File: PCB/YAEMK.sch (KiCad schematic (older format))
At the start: 81 parts, among them SW1 ALPS EC11

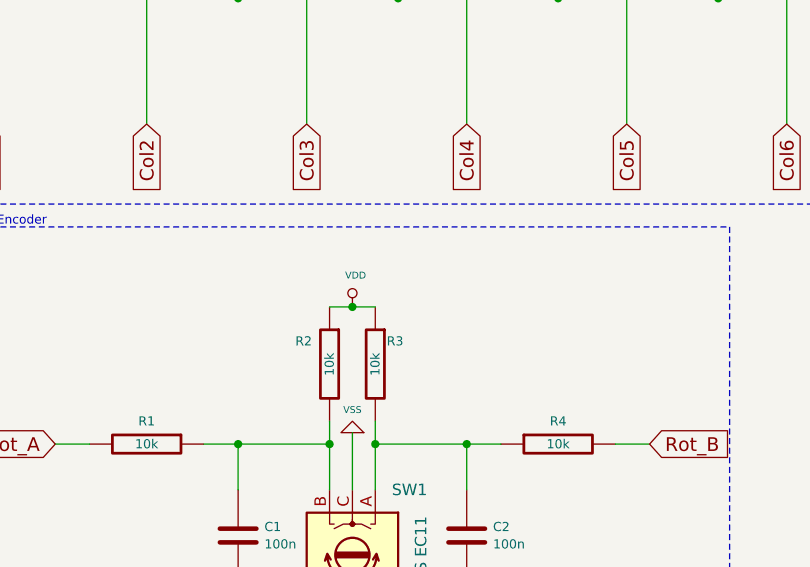
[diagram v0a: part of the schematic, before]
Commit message: YAEMK 1.2 RC
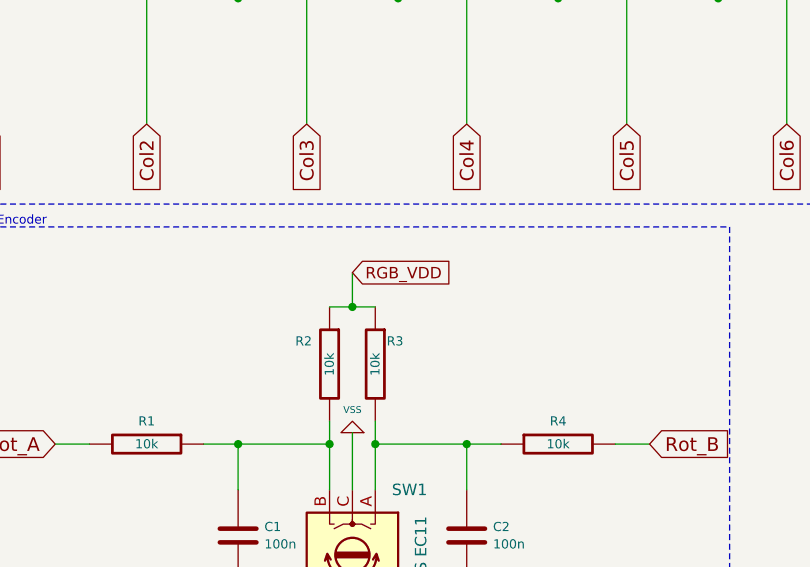
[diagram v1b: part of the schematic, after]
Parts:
- D1, D10, D11, D12, D13, D14, D15, D16, D17, D18, D19, D2, D20, D21, D22, D23, D24, D25, D26, D27, D28, D29, D3, D30, D31, D32, D33, D34, D4, D5, D6, D7, D8, D9: footprint Diode_SMD:D_SOD-523 -> prettylib:D_SOD-523
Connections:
- net VDD renamed RGB_VDD
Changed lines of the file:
@@
 F 0 "D3" H 1800 1150 40  0000 C CNN
 F 1 "DIODE" H 1800 950 40  0000 C CNN
-F 2 "Diode_SMD:D_SOD-523" H 1800 1050 60  0001 C CNN
+F 2 "prettylib:D_SOD-523" H 1800 1050 60  0001 C CNN
 F 3 "~" H 1800 1050 60  0000 C CNN
 	1    1800 1050
@@
 F 0 "D8" H 2500 1150 40  0000 C CNN
 F 1 "DIODE" H 2500 950 40  0000 C CNN
-F 2 "Diode_SMD:D_SOD-523" H 2500 1050 60  0001 C CNN
+F 2 "prettylib:D_SOD-523" H 2500 1050 60  0001 C CNN
 F 3 "~" H 2500 1050 60  0000 C CNN
 	1    2500 1050
@@
 F 0 "D13" H 3200 1150 40  0000 C CNN
 F 1 "DIODE" H 3200 950 40  0000 C CNN
-F 2 "Diode_SMD:D_SOD-523" H 3200 1050 60  0001 C CNN
+F 2 "prettylib:D_SOD-523" H 3200 1050 60  0001 C CNN
 F 3 "~" H 3200 1050 60  0000 C CNN
 	1    3200 1050
@@
 F 0 "D18" H 3900 1150 40  0000 C CNN
 F 1 "DIODE" H 3900 950 40  0000 C CNN
-F 2 "Diode_SMD:D_SOD-523" H 3900 1050 60  0001 C CNN
+F 2 "prettylib:D_SOD-523" H 3900 1050 60  0001 C CNN
 F 3 "~" H 3900 1050 60  0000 C CNN
 	1    3900 1050
@@
 F 0 "D23" H 4600 1150 40  0000 C CNN
 F 1 "DIODE" H 4600 950 40  0000 C CNN
-F 2 "Diode_SMD:D_SOD-523" H 4600 1050 60  0001 C CNN
+F 2 "prettylib:D_SOD-523" H 4600 1050 60  0001 C CNN
 F 3 "~" H 4600 1050 60  0000 C CNN
 	1    4600 1050
@@
 F 0 "D27" H 5300 1150 40  0000 C CNN
 F 1 "DIODE" H 5300 950 40  0000 C CNN
-F 2 "Diode_SMD:D_SOD-523" H 5300 1050 60  0001 C CNN
+F 2 "prettylib:D_SOD-523" H 5300 1050 60  0001 C CNN
 F 3 "~" H 5300 1050 60  0000 C CNN
 	1    5300 1050
@@
 F 0 "D31" H 6000 1150 40  0000 C CNN
 F 1 "DIODE" H 6000 950 40  0000 C CNN
-F 2 "Diode_SMD:D_SOD-523" H 6000 1050 60  0001 C CNN
+F 2 "prettylib:D_SOD-523" H 6000 1050 60  0001 C CNN
 F 3 "~" H 6000 1050 60  0000 C CNN
 	1    6000 1050
@@
 F 0 "D4" H 1800 1850 40  0000 C CNN
 F 1 "DIODE" H 1800 1650 40  0000 C CNN
-F 2 "Diode_SMD:D_SOD-523" H 1800 1750 60  0001 C CNN
+F 2 "prettylib:D_SOD-523" H 1800 1750 60  0001 C CNN
 F 3 "~" H 1800 1750 60  0000 C CNN
 	1    1800 1750
@@
 F 0 "D9" H 2500 1850 40  0000 C CNN
 F 1 "DIODE" H 2500 1650 40  0000 C CNN
-F 2 "Diode_SMD:D_SOD-523" H 2500 1750 60  0001 C CNN
+F 2 "prettylib:D_SOD-523" H 2500 1750 60  0001 C CNN
 F 3 "~" H 2500 1750 60  0000 C CNN
 	1    2500 1750
@@
 F 0 "D14" H 3200 1850 40  0000 C CNN
 F 1 "DIODE" H 3200 1650 40  0000 C CNN
-F 2 "Diode_SMD:D_SOD-523" H 3200 1750 60  0001 C CNN
+F 2 "prettylib:D_SOD-523" H 3200 1750 60  0001 C CNN
 F 3 "~" H 3200 1750 60  0000 C CNN
 	1    3200 1750
@@
 F 0 "D19" H 3900 1850 40  0000 C CNN
 F 1 "DIODE" H 3900 1650 40  0000 C CNN
-F 2 "Diode_SMD:D_SOD-523" H 3900 1750 60  0001 C CNN
+F 2 "prettylib:D_SOD-523" H 3900 1750 60  0001 C CNN
 F 3 "~" H 3900 1750 60  0000 C CNN
 	1    3900 1750
@@
 F 0 "D24" H 4600 1850 40  0000 C CNN
 F 1 "DIODE" H 4600 1650 40  0000 C CNN
-F 2 "Diode_SMD:D_SOD-523" H 4600 1750 60  0001 C CNN
+F 2 "prettylib:D_SOD-523" H 4600 1750 60  0001 C CNN
 F 3 "~" H 4600 1750 60  0000 C CNN
 	1    4600 1750
@@
 F 0 "D28" H 5300 1850 40  0000 C CNN
 F 1 "DIODE" H 5300 1650 40  0000 C CNN
-F 2 "Diode_SMD:D_SOD-523" H 5300 1750 60  0001 C CNN
+F 2 "prettylib:D_SOD-523" H 5300 1750 60  0001 C CNN
 F 3 "~" H 5300 1750 60  0000 C CNN
 	1    5300 1750
@@
 F 0 "D32" H 6000 1850 40  0000 C CNN
 F 1 "DIODE" H 6000 1650 40  0000 C CNN
-F 2 "Diode_SMD:D_SOD-523" H 6000 1750 60  0001 C CNN
+F 2 "prettylib:D_SOD-523" H 6000 1750 60  0001 C CNN
 F 3 "~" H 6000 1750 60  0000 C CNN
 	1    6000 1750
@@
 F 0 "D10" H 2500 2550 40  0000 C CNN
 F 1 "DIODE" H 2500 2350 40  0000 C CNN
-F 2 "Diode_SMD:D_SOD-523" H 2500 2450 60  0001 C CNN
+F 2 "prettylib:D_SOD-523" H 2500 2450 60  0001 C CNN
 F 3 "~" H 2500 2450 60  0000 C CNN
 	1    2500 2450
@@
 F 0 "D15" H 3200 2550 40  0000 C CNN
 F 1 "DIODE" H 3200 2350 40  0000 C CNN
-F 2 "Diode_SMD:D_SOD-523" H 3200 2450 60  0001 C CNN
+F 2 "prettylib:D_SOD-523" H 3200 2450 60  0001 C CNN
 F 3 "~" H 3200 2450 60  0000 C CNN
 	1    3200 2450
@@
 F 0 "D20" H 3900 2550 40  0000 C CNN
 F 1 "DIODE" H 3900 2350 40  0000 C CNN
-F 2 "Diode_SMD:D_SOD-523" H 3900 2450 60  0001 C CNN
+F 2 "prettylib:D_SOD-523" H 3900 2450 60  0001 C CNN
 F 3 "~" H 3900 2450 60  0000 C CNN
 	1    3900 2450
@@
 F 0 "D25" H 4600 2550 40  0000 C CNN
 F 1 "DIODE" H 4600 2350 40  0000 C CNN
-F 2 "Diode_SMD:D_SOD-523" H 4600 2450 60  0001 C CNN
+F 2 "prettylib:D_SOD-523" H 4600 2450 60  0001 C CNN
 F 3 "~" H 4600 2450 60  0000 C CNN
 	1    4600 2450
@@
 F 0 "D29" H 5300 2550 40  0000 C CNN
 F 1 "DIODE" H 5300 2350 40  0000 C CNN
-F 2 "Diode_SMD:D_SOD-523" H 5300 2450 60  0001 C CNN
+F 2 "prettylib:D_SOD-523" H 5300 2450 60  0001 C CNN
 F 3 "~" H 5300 2450 60  0000 C CNN
 	1    5300 2450
@@
 F 0 "D33" H 6000 2550 40  0000 C CNN
 F 1 "DIODE" H 6000 2350 40  0000 C CNN
-F 2 "Diode_SMD:D_SOD-523" H 6000 2450 60  0001 C CNN
+F 2 "prettylib:D_SOD-523" H 6000 2450 60  0001 C CNN
 F 3 "~" H 6000 2450 60  0000 C CNN
 	1    6000 2450
@@
 F 0 "D1" H 1100 3250 40  0000 C CNN
 F 1 "DIODE" H 1100 3050 40  0000 C CNN
-F 2 "Diode_SMD:D_SOD-523" H 1100 3150 60  0001 C CNN
+F 2 "prettylib:D_SOD-523" H 1100 3150 60  0001 C CNN
 F 3 "~" H 1100 3150 60  0000 C CNN
 	1    1100 3150
@@
 F 0 "D6" H 1800 3250 40  0000 C CNN
 F 1 "DIODE" H 1800 3050 40  0000 C CNN
-F 2 "Diode_SMD:D_SOD-523" H 1800 3150 60  0001 C CNN
+F 2 "prettylib:D_SOD-523" H 1800 3150 60  0001 C CNN
 F 3 "~" H 1800 3150 60  0000 C CNN
 	1    1800 3150
@@
 F 0 "D11" H 2500 3250 40  0000 C CNN
 F 1 "DIODE" H 2500 3050 40  0000 C CNN
-F 2 "Diode_SMD:D_SOD-523" H 2500 3150 60  0001 C CNN
+F 2 "prettylib:D_SOD-523" H 2500 3150 60  0001 C CNN
 F 3 "~" H 2500 3150 60  0000 C CNN
 	1    2500 3150
@@
 F 0 "D16" H 3200 3250 40  0000 C CNN
 F 1 "DIODE" H 3200 3050 40  0000 C CNN
-F 2 "Diode_SMD:D_SOD-523" H 3200 3150 60  0001 C CNN
+F 2 "prettylib:D_SOD-523" H 3200 3150 60  0001 C CNN
 F 3 "~" H 3200 3150 60  0000 C CNN
 	1    3200 3150
@@
 F 0 "D21" H 3900 3250 40  0000 C CNN
 F 1 "DIODE" H 3900 3050 40  0000 C CNN
-F 2 "Diode_SMD:D_SOD-523" H 3900 3150 60  0001 C CNN
+F 2 "prettylib:D_SOD-523" H 3900 3150 60  0001 C CNN
 F 3 "~" H 3900 3150 60  0000 C CNN
 	1    3900 3150
@@
 F 0 "D26" H 4600 3250 40  0000 C CNN
 F 1 "DIODE" H 4600 3050 40  0000 C CNN
-F 2 "Diode_SMD:D_SOD-523" H 4600 3150 60  0001 C CNN
+F 2 "prettylib:D_SOD-523" H 4600 3150 60  0001 C CNN
 F 3 "~" H 4600 3150 60  0000 C CNN
 	1    4600 3150
@@
 F 0 "D30" H 5300 3250 40  0000 C CNN
 F 1 "DIODE" H 5300 3050 40  0000 C CNN
-F 2 "Diode_SMD:D_SOD-523" H 5300 3150 60  0001 C CNN
+F 2 "prettylib:D_SOD-523" H 5300 3150 60  0001 C CNN
 F 3 "~" H 5300 3150 60  0000 C CNN
 	1    5300 3150
@@
 F 0 "D34" H 6000 3250 40  0000 C CNN
 F 1 "DIODE" H 6000 3050 40  0000 C CNN
-F 2 "Diode_SMD:D_SOD-523" H 6000 3150 60  0001 C CNN
+F 2 "prettylib:D_SOD-523" H 6000 3150 60  0001 C CNN
 F 3 "~" H 6000 3150 60  0000 C CNN
 	1    6000 3150
@@
 F 0 "D2" H 1100 3950 40  0000 C CNN
 F 1 "DIODE" H 1100 3750 40  0000 C CNN
-F 2 "Diode_SMD:D_SOD-523" H 1100 3850 60  0001 C CNN
+F 2 "prettylib:D_SOD-523" H 1100 3850 60  0001 C CNN
 F 3 "~" H 1100 3850 60  0000 C CNN
 	1    1100 3850
@@
 F 0 "D7" H 1800 3950 40  0000 C CNN
 F 1 "DIODE" H 1800 3750 40  0000 C CNN
-F 2 "Diode_SMD:D_SOD-523" H 1800 3850 60  0001 C CNN
+F 2 "prettylib:D_SOD-523" H 1800 3850 60  0001 C CNN
 F 3 "~" H 1800 3850 60  0000 C CNN
 	1    1800 3850
@@
 F 0 "D12" H 2500 3950 40  0000 C CNN
 F 1 "DIODE" H 2500 3750 40  0000 C CNN
-F 2 "Diode_SMD:D_SOD-523" H 2500 3850 60  0001 C CNN
+F 2 "prettylib:D_SOD-523" H 2500 3850 60  0001 C CNN
 F 3 "~" H 2500 3850 60  0000 C CNN
 	1    2500 3850
@@
 F 0 "D17" H 3200 3950 40  0000 C CNN
 F 1 "DIODE" H 3200 3750 40  0000 C CNN
-F 2 "Diode_SMD:D_SOD-523" H 3200 3850 60  0001 C CNN
+F 2 "prettylib:D_SOD-523" H 3200 3850 60  0001 C CNN
 F 3 "~" H 3200 3850 60  0000 C CNN
 	1    3200 3850
@@
 F 0 "D5" H 1800 2550 40  0000 C CNN
 F 1 "DIODE" H 1800 2350 40  0000 C CNN
-F 2 "Diode_SMD:D_SOD-523" H 1800 2450 60  0001 C CNN
+F 2 "prettylib:D_SOD-523" H 1800 2450 60  0001 C CNN
 F 3 "~" H 1800 2450 60  0000 C CNN
 	1    1800 2450
@@
 F 0 "D22" H 3900 3950 40  0000 C CNN
 F 1 "DIODE" H 3900 3750 40  0000 C CNN
-F 2 "Diode_SMD:D_SOD-523" H 3900 3850 60  0001 C CNN
+F 2 "prettylib:D_SOD-523" H 3900 3850 60  0001 C CNN
 F 3 "~" H 3900 3850 60  0000 C CNN
 	1    3900 3850
@@
 Wire Wire Line
 	2200 5400 2300 5400
-$Comp
-L YAEMK:VDD #PWR02
-U 1 1 5FA3B535
-P 2300 5400
-F 0 "#PWR02" H 2300 5500 30  0001 C CNN
-F 1 "VDD" H 2314 5538 30  0000 C CNN
-F 2 "" H 2300 5400 60  0000 C CNN
-F 3 "" H 2300 5400 60  0000 C CNN
-	1    2300 5400
-	1    0    0    -1
-$EndComp
+Text GLabel 2300 5250 2    50   Input ~ 0
+RGB_VDD
+Wire Wire Line
+	2300 5250 2300 5400
 Connection ~ 2300 5400
 Wire Wire Line

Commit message: Clean up save point
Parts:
- MH1, MH2, MH3, MH4, MH5, MH6, MH7, MH8, MH9: symbol YAEMK-rescue:Mounting_Hole-YAEMK -> YAEMK:Mounting_Hole
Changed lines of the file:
@@
 Wire Wire Line
 	5600 2250 5600 2950
-Wire Wire Line
-	5600 1550 5600 2250
 $Sheet
 S 8450 650  850  800
@@
 Text Notes 550  600  0    39   ~ 0
 Switch Matrix
-$Sheet
-S 8450 1800 850  850
-U 549878F0
-F0 "mcu" 50
-F1 "mcu.sch" 50
-$EndSheet
 $Comp
 L YAEMK:MX_WS2812_2U_2X1U S1
@@
 Rot_Row
 $Comp
-L YAEMK-rescue:Mounting_Hole-YAEMK MH6
+L YAEMK:Mounting_Hole MH6
 U 1 1 5EF9B2DD
 P 7900 2400
@@
 $EndComp
 $Comp
-L YAEMK-rescue:Mounting_Hole-YAEMK MH1
+L YAEMK:Mounting_Hole MH1
 U 1 1 5EF9B5B8
 P 7900 800
@@
 $EndComp
 $Comp
-L YAEMK-rescue:Mounting_Hole-YAEMK MH7
+L YAEMK:Mounting_Hole MH7
 U 1 1 5EF9C683
 P 7900 2700
@@
 $EndComp
 $Comp
-L YAEMK-rescue:Mounting_Hole-YAEMK MH2
+L YAEMK:Mounting_Hole MH2
 U 1 1 5EF9D40E
 P 7900 1100
@@
 $EndComp
 $Comp
-L YAEMK-rescue:Mounting_Hole-YAEMK MH8
+L YAEMK:Mounting_Hole MH8
 U 1 1 5EF9E2EE
 P 7900 3000
@@
 $EndComp
 $Comp
-L YAEMK-rescue:Mounting_Hole-YAEMK MH3
+L YAEMK:Mounting_Hole MH3
 U 1 1 5EF9E2F8
 P 7900 1400
@@
 $EndComp
 $Comp
-L YAEMK-rescue:Mounting_Hole-YAEMK MH9
+L YAEMK:Mounting_Hole MH9
 U 1 1 5EF9E302
 P 7900 3300
@@
 $EndComp
 $Comp
-L YAEMK-rescue:Mounting_Hole-YAEMK MH4
+L YAEMK:Mounting_Hole MH4
 U 1 1 5EF9E30C
 P 7900 1700
@@
 $EndComp
 $Comp
-L YAEMK-rescue:Mounting_Hole-YAEMK MH5
+L YAEMK:Mounting_Hole MH5
 U 1 1 5F03D0F0
 P 7900 2050
@@
 	0    1    1    0
 $EndComp
-Wire Wire Line
-	7800 800  7800 1100
-Connection ~ 7800 1100
-Wire Wire Line
-	7800 1100 7800 1400
-Connection ~ 7800 1400
-Wire Wire Line
-	7800 1400 7800 1700
-Connection ~ 7800 1700
-Wire Wire Line
-	7800 1700 7800 2050
-Connection ~ 7800 2050
-Wire Wire Line
-	7800 2050 7800 2400
-Connection ~ 7800 2400
-Wire Wire Line
-	7800 2400 7800 2700
-Connection ~ 7800 2700
-Wire Wire Line
-	7800 2700 7800 3000
-Connection ~ 7800 3000
-Wire Wire Line
-	7800 3000 7800 3300
 $Comp
 L YAEMK:VSS #PWR05
@@
 $EndComp
 Wire Wire Line
-	7800 3300 7800 3600
-Connection ~ 7800 3300
-Wire Wire Line
 	3500 2950 3500 4600
 Wire Notes Line
@@
 Wire Wire Line
 	2300 5400 2400 5400
+Wire Wire Line
+	7800 800  7800 1100
+Connection ~ 7800 1100
+Wire Wire Line
+	7800 1100 7800 1400
+Connection ~ 7800 1400
+Wire Wire Line
+	7800 1400 7800 1700
+Connection ~ 7800 1700
+Wire Wire Line
+	7800 1700 7800 2050
+Connection ~ 7800 2050
+Wire Wire Line
+	7800 2050 7800 2400
+Connection ~ 7800 2400
+Wire Wire Line
+	7800 2400 7800 2700
+Connection ~ 7800 2700
+Wire Wire Line
+	7800 2700 7800 3000
+Connection ~ 7800 3000
+Wire Wire Line
+	7800 3000 7800 3300
+Connection ~ 7800 3300
+Wire Wire Line
+	7800 3300 7800 3600
+$Sheet
+S 8450 1800 850  850
+U 549878F0
+F0 "mcu" 50
+F1 "mcu.sch" 50
+$EndSheet
+Wire Wire Line
+	5600 1550 5600 2250
 $EndSCHEMATC
